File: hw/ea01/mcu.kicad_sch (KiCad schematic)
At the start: 44 parts, among them J2 USB_B, J3 Conn_01x05_Pin, J8 Conn_01x03_Pin, J9 Conn_01x03_Pin, SW1 SW_Push, SW2 SW_Push, U1 RP2040, U11 W25Q32JVSS, U3 NUP2202, Y1 12Mhz

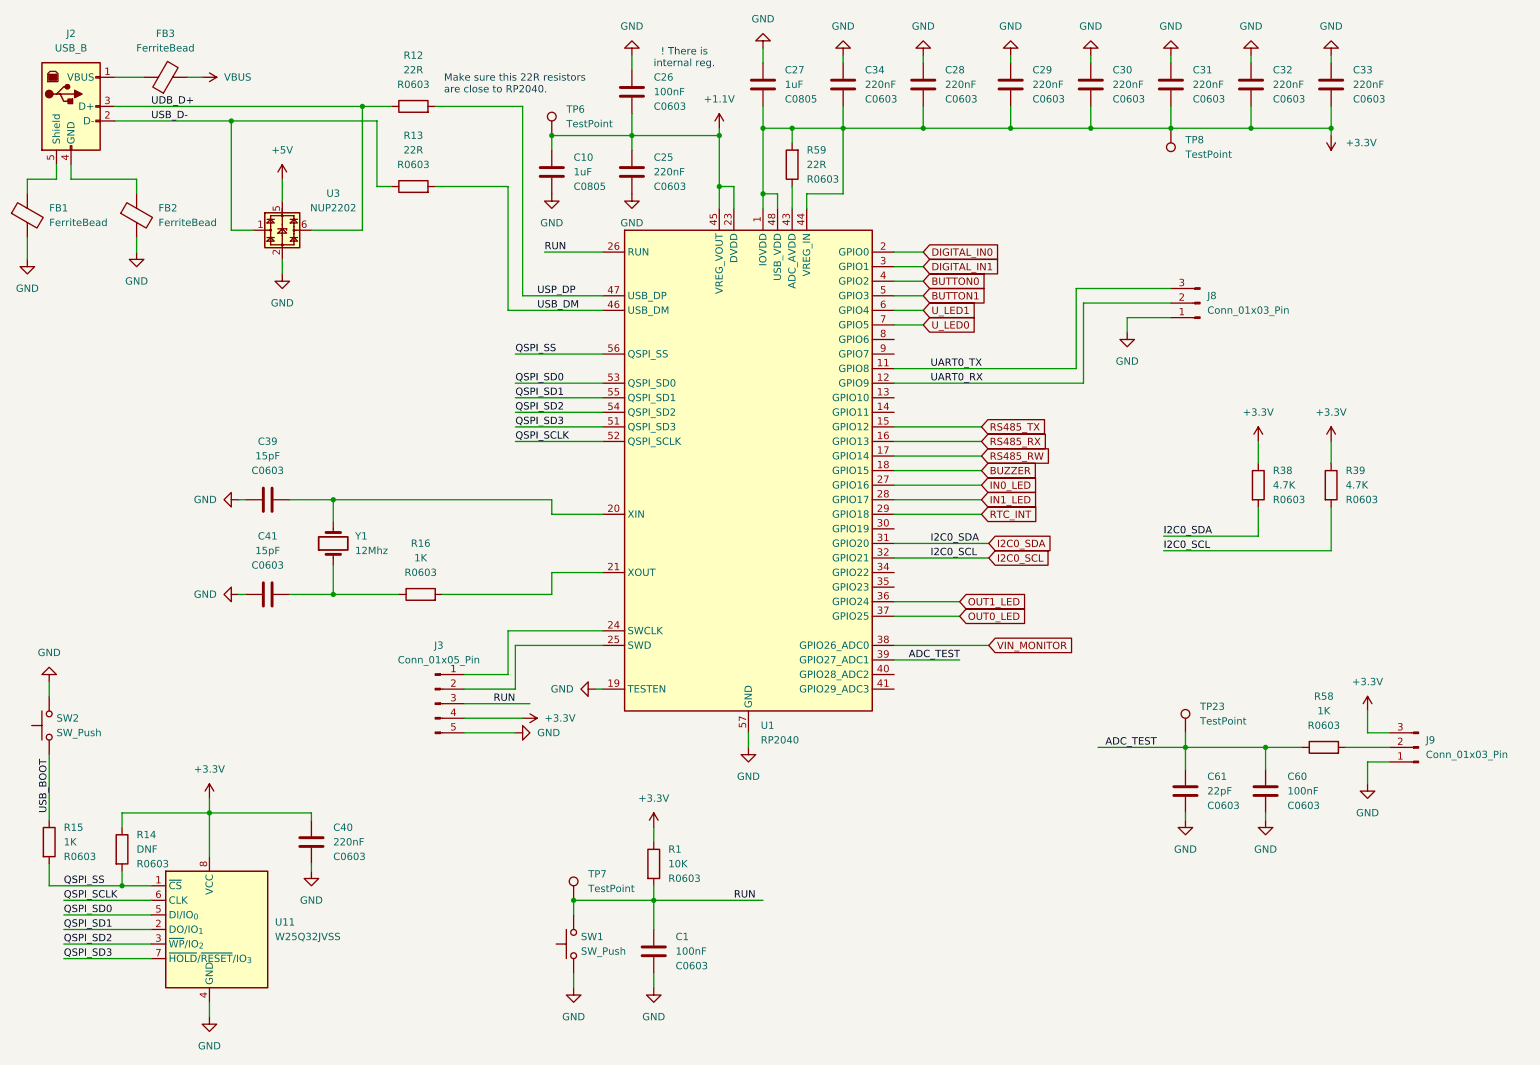
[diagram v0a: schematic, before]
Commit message: pcb drawing continue..
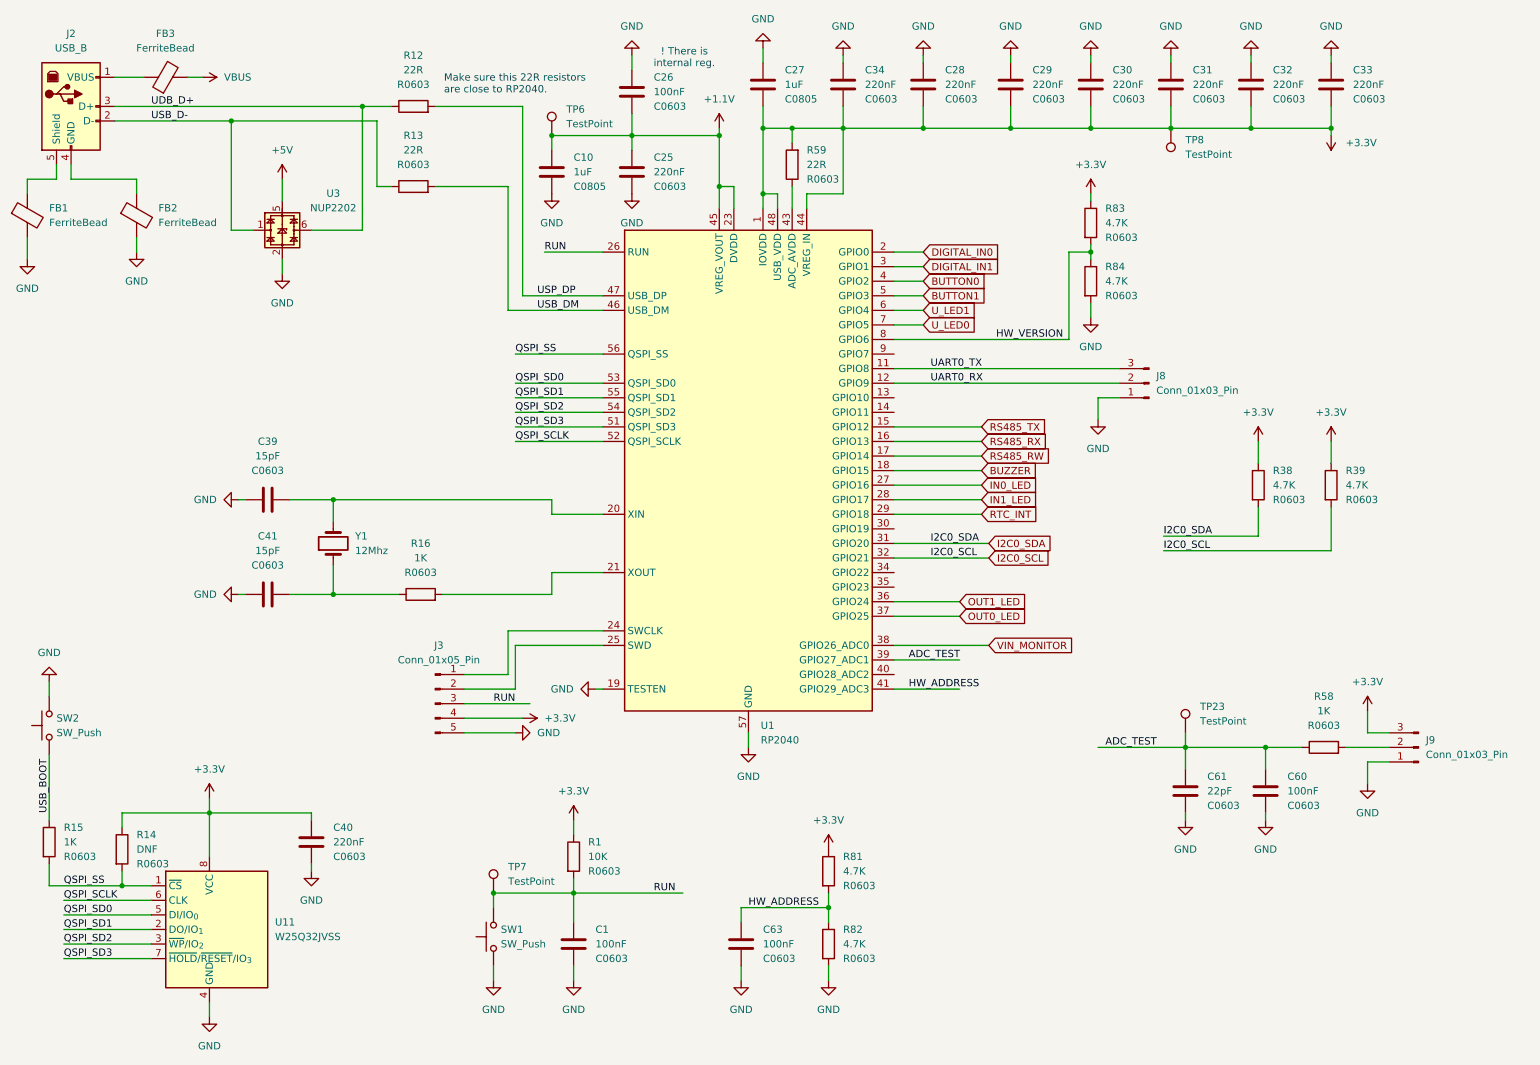
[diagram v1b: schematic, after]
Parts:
- added C63: 100nF, Capacitor_SMD:C_0603_1608Metric, symbol Device:C
- added R81, R82, R83, R84: 4.7K, Resistor_SMD:R_0603_1608Metric, symbol Device:R
- SW1, SW2: footprint Button_Switch_THT:SW_PUSH_6mm_H5mm -> Button_Switch_THT:SW_Tactile_SPST_Angled_PTS645Vx83-2LFS
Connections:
- net +3.3V: now also R81.1, R83.1
- net GND: now also C63.2, R82.2, R84.2
- net HW_ADDRESS: now reaches U1.41 (GPIO29_ADC3)
- net HW_ADDRESS: now also C63.1, R81.2, R82.1
- net HW_VERSION: now reaches U1.8 (GPIO6)
- net HW_VERSION: now also R83.2, R84.1
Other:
- moved on the sheet: C1, J8, R1, SW1, TP7
